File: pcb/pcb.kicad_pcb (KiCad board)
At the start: 2 copper layers, 75 x 75 mm, 4 parts, among them U1 1117-3.3

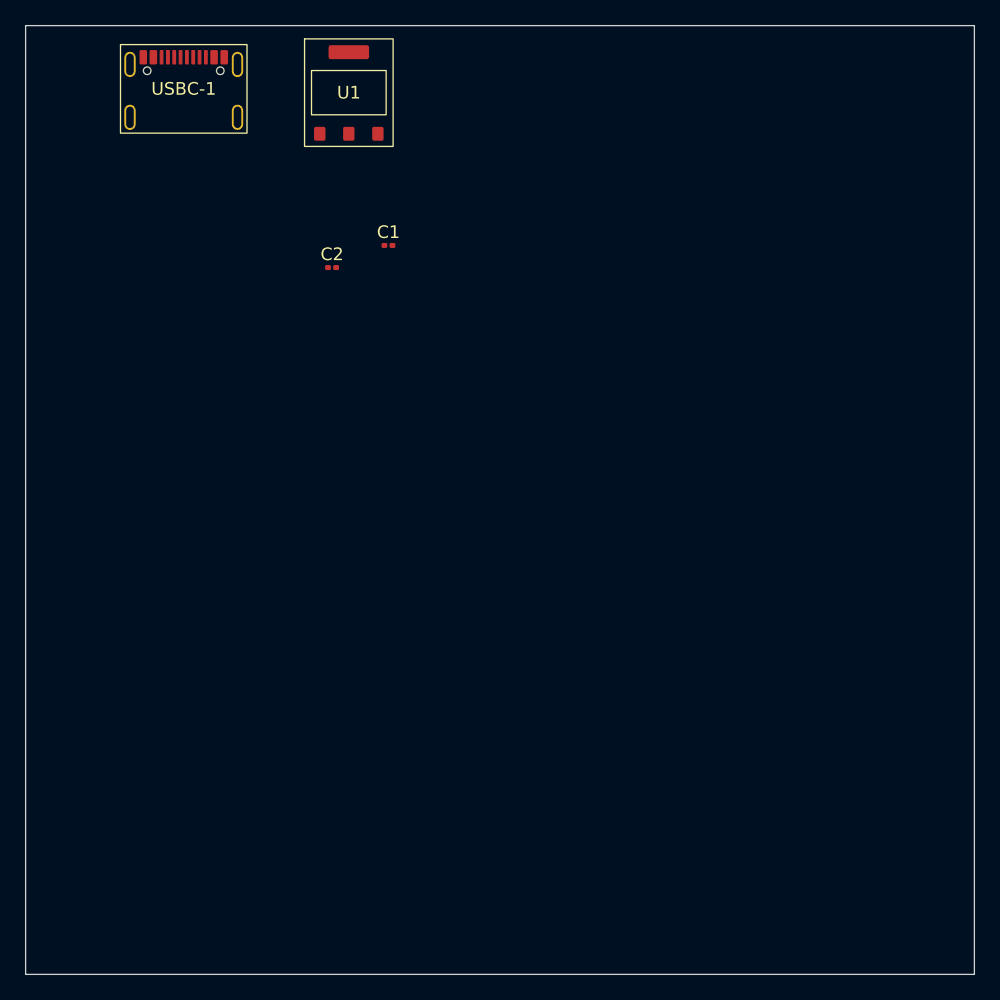
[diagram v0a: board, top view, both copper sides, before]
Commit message: wired some stuff
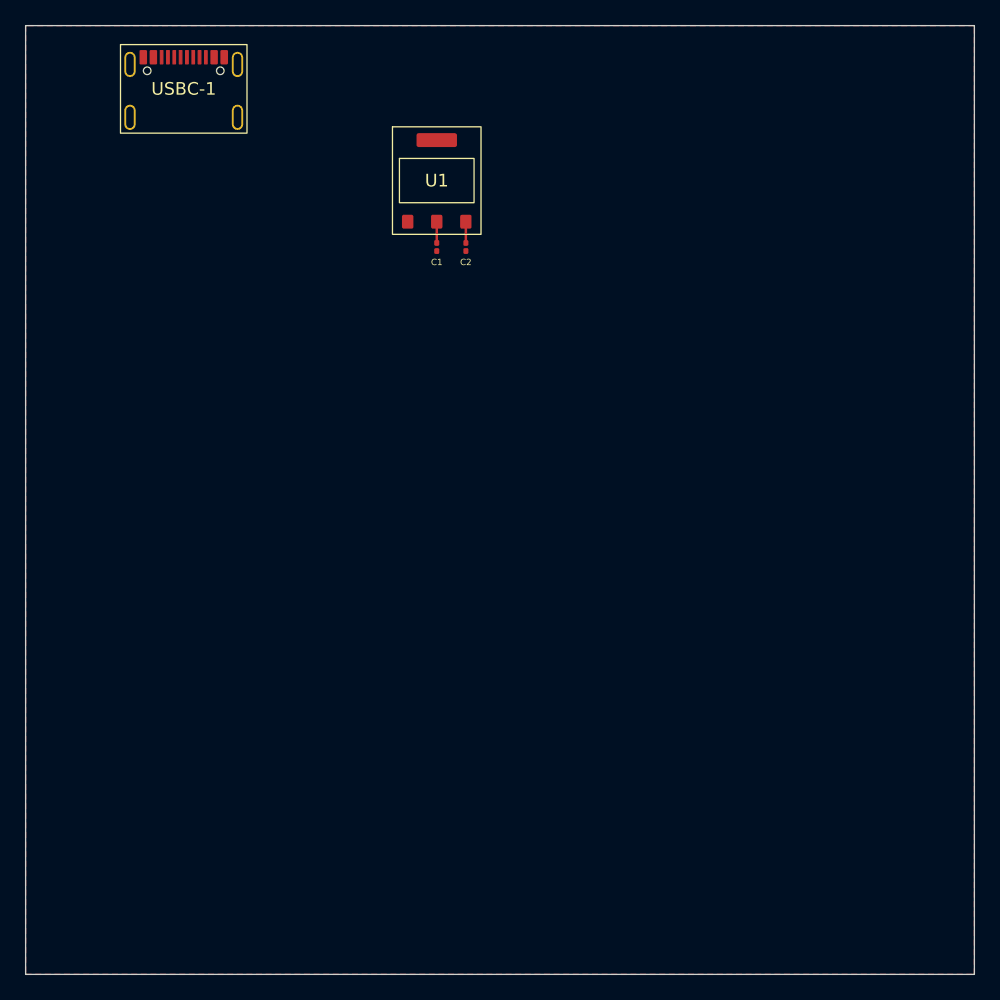
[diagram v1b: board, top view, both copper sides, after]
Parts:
- moved C2 10.7 mm to (34.8, 17.5), turned to -90 degrees
- moved U1 9.83 mm to (32.5, 15.5)
- moved C1 3.82 mm to (32.5, 17.5), turned to 90 degrees
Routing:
- net VBUS: track 0.00 -> 1.68 mm
- net Net-(U1-VIN): track 0.00 -> 1.68 mm
- added copper zone on F.Cu, net GND
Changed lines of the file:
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@@
 	(footprint "Capacitor_SMD:C_0201_0603Metric"
 		(layer "F.Cu")
-		(at 28.68 17.375)
+		(at 32.5 17.5 90)
 		(descr "Capacitor SMD 0201 (0603 Metric), square (rectangular) end terminal, IPC-7351 nominal, (Body size source: https://www.vishay.com/docs/20052/crcw0201e3.pdf)")
 		(tags "capacitor")
 		(property "Reference" "C1"
-			(at 0 -1.05 0)
-			(layer "F.SilkS")
-			(effects
-				(font
-					(size 1 1)
-					(thickness 0.15)
+			(at -1.2 0 180)
+			(layer "F.SilkS")
+			(effects
+				(font
+					(size 0.5 0.5)
+					(thickness 0.125)
 				)
 			)
 		)
 		(property "Value" "10uF"
-			(at 0 1.05 0)
-			(layer "F.Fab")
-			(effects
-				(font
-					(size 1 1)
-					(thickness 0.15)
+			(at 0 1.05 90)
+			(layer "F.Fab")
+			(hide yes)
+			(effects
+				(font
+					(size 0.5 0.5)
+					(thickness 0.125)
 				)
 			)
 		)
 		(property "Datasheet" ""
-			(at 0 0 0)
+			(at 0 0 90)
 			(layer "F.Fab")
 			(hide yes)
@@
 		)
 		(property "Description" "Unpolarized capacitor"
-			(at 0 0 0)
+			(at 0 0 90)
 			(layer "F.Fab")
 			(hide yes)
@@
 		)
 		(property "KiLib_Generator" "SMD_2terminal_chip_molded"
-			(at 0 0 0)
+			(at 0 0 90)
 			(layer "F.SilkS")
 			(hide yes)
@@
 		)
 		(property "LCSC" "C1691"
-			(at 0 0 0)
+			(at 0 0 90)
 			(unlocked yes)
 			(layer "F.Fab")
@@
 		)
 		(fp_text user "${REFERENCE}"
-			(at 0 -0.68 0)
+			(at 0 0 90)
 			(layer "F.Fab")
 			(effects
@@
 		)
 		(pad "" smd roundrect
-			(at -0.345 0)
+			(at -0.345 0 90)
 			(size 0.318 0.36)
 			(layers "F.Paste")
@@
 		)
 		(pad "" smd roundrect
-			(at 0.345 0)
+			(at 0.345 0 90)
 			(size 0.318 0.36)
 			(layers "F.Paste")
@@
 		)
 		(pad "1" smd roundrect
-			(at -0.32 0)
+			(at -0.32 0 90)
 			(size 0.46 0.4)
 			(layers "F.Cu" "F.Mask")
@@
 		)
 		(pad "2" smd roundrect
-			(at 0.32 0)
+			(at 0.32 0 90)
 			(size 0.46 0.4)
 			(layers "F.Cu" "F.Mask")
@@
 	(footprint "Andrews_Library:LCSC_SMD_1117-3.3v_C5125088"
 		(layer "F.Cu")
-		(at 25.55 8.55)
+		(at 32.5 15.5)
 		(property "Reference" "U1"
 			(at 0 -3.25 0)
@@
 		)
 		(property "Value" "1117-3.3"
-			(at 0 3.9 0)
+			(at 0 -8.7 0)
 			(unlocked yes)
 			(layer "F.Fab")
@@
 		)
 		(fp_text user "${REFERENCE}"
-			(at 0 2.1 0)
+			(at 0 -10.5 0)
 			(unlocked yes)
 			(layer "F.Fab")
@@
 			(polygon
 				(pts
-					(xy 22.05 1.05) (xy 29.05 1.05) (xy 29.05 9.55) (xy 22.05 9.55)
+					(xy 29 8) (xy 36 8) (xy 36 16.5) (xy 29 16.5)
 				)
 			)
@@
 	(footprint "Capacitor_SMD:C_0201_0603Metric"
 		(layer "F.Cu")
-		(at 24.225 19.125)
+		(at 34.8 17.5 -90)
 		(descr "Capacitor SMD 0201 (0603 Metric), square (rectangular) end terminal, IPC-7351 nominal, (Body size source: https://www.vishay.com/docs/20052/crcw0201e3.pdf)")
 		(tags "capacitor")
 		(property "Reference" "C2"
-			(at 0 -1.05 0)
-			(layer "F.SilkS")
-			(effects
-				(font
-					(size 1 1)
-					(thickness 0.15)
+			(at 1.2 0 0)
+			(layer "F.SilkS")
+			(effects
+				(font
+					(size 0.5 0.5)
+					(thickness 0.125)
 				)
 			)
 		)
 		(property "Value" "10uF"
-			(at 0 1.05 0)
-			(layer "F.Fab")
-			(effects
-				(font
-					(size 1 1)
-					(thickness 0.15)
+			(at 0 1.05 90)
+			(layer "F.Fab")
+			(hide yes)
+			(effects
+				(font
+					(size 0.5 0.5)
+					(thickness 0.125)
 				)
 			)
 		)
 		(property "Datasheet" ""
-			(at 0 0 0)
+			(at 0 0 90)
 			(layer "F.Fab")
 			(hide yes)
@@
 		)
 		(property "Description" "Unpolarized capacitor"
-			(at 0 0 0)
+			(at 0 0 90)
 			(layer "F.Fab")
 			(hide yes)
@@
 		)
 		(property "KiLib_Generator" "SMD_2terminal_chip_molded"
-			(at 0 0 0)
+			(at 0 0 90)
 			(layer "F.SilkS")
 			(hide yes)
@@
 		)
 		(property "LCSC" "C1691"
-			(at 0 0 0)
+			(at 0 0 270)
 			(unlocked yes)
 			(layer "F.Fab")
@@
 		)
 		(fp_text user "${REFERENCE}"
-			(at 0 -0.68 0)
+			(at 0 -0.05 90)
 			(layer "F.Fab")
 			(effects
@@
 		)
 		(pad "" smd roundrect
-			(at -0.345 0)
+			(at -0.345 0 270)
 			(size 0.318 0.36)
 			(layers "F.Paste")
@@
 		)
 		(pad "" smd roundrect
-			(at 0.345 0)
+			(at 0.345 0 270)
 			(size 0.318 0.36)
 			(layers "F.Paste")
@@
 		)
 		(pad "1" smd roundrect
-			(at -0.32 0)
+			(at -0.32 0 270)
 			(size 0.46 0.4)
 			(layers "F.Cu" "F.Mask")
@@
 		)
 		(pad "2" smd roundrect
-			(at 0.32 0)
+			(at 0.32 0 270)
 			(size 0.46 0.4)
 			(layers "F.Cu" "F.Mask")
@@
 		(layer "Edge.Cuts")
 	)
+	(segment
+		(start 32.5 15.5)
+		(end 32.5 17.18)
+		(width 0.2)
+		(layer "F.Cu")
+		(net "VBUS")
+	)
+	(segment
+		(start 34.8 15.5)
+		(end 34.8 17.18)
+		(width 0.2)
+		(layer "F.Cu")
+		(net "Net-(U1-VIN)")
+	)
+	(zone
+		(net "GND")
+		(layer "F.Cu")
+		(hatch edge 0.5)
+		(connect_pads
+			(clearance 0.5)
+		)
+		(min_thickness 0.25)
+		(fill yes
+			(thermal_gap 0.5)
+			(thermal_bridge_width 0.5)
+			(island_removal_mode 0)
+		)
+		(polygon
+			(pts
+				(xy 75 0) (xy 0 0) (xy 0 75) (xy 75 75)
+			)
+		)
+	)
+	(group ""
+		(members "4c363494-5d20-44a3-9b12-37bc64127a15" "7ff470fd-2abd-486a-b746-3b467e71a7f8"
+			"a43b688b-cef3-4c08-969a-ef6623efc0b7" "c16a55e6-c9ba-4bf5-9418-845e8fc3c2c0"
+			"e2951551-5bd3-452b-943a-e5c31ddf3bfe"
+		)
+	)
 	(embedded_fonts no)
